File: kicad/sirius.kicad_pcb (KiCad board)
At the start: 4 copper layers, 31.2 x 65.4 mm, 56 parts, among them J1 IPEX_MHF1, J2 Power In, J3 Screw_Terminal, Q1 Q_PMOS_GSD, Q2 Q_NMOS_GSD, Q3 Q_NMOS_GSD, U1 Power_Connector, U2 AP63301WU-7, U3 RFM95W-915S2, U4 LC29H (DA), U5 Pi Zero 2W

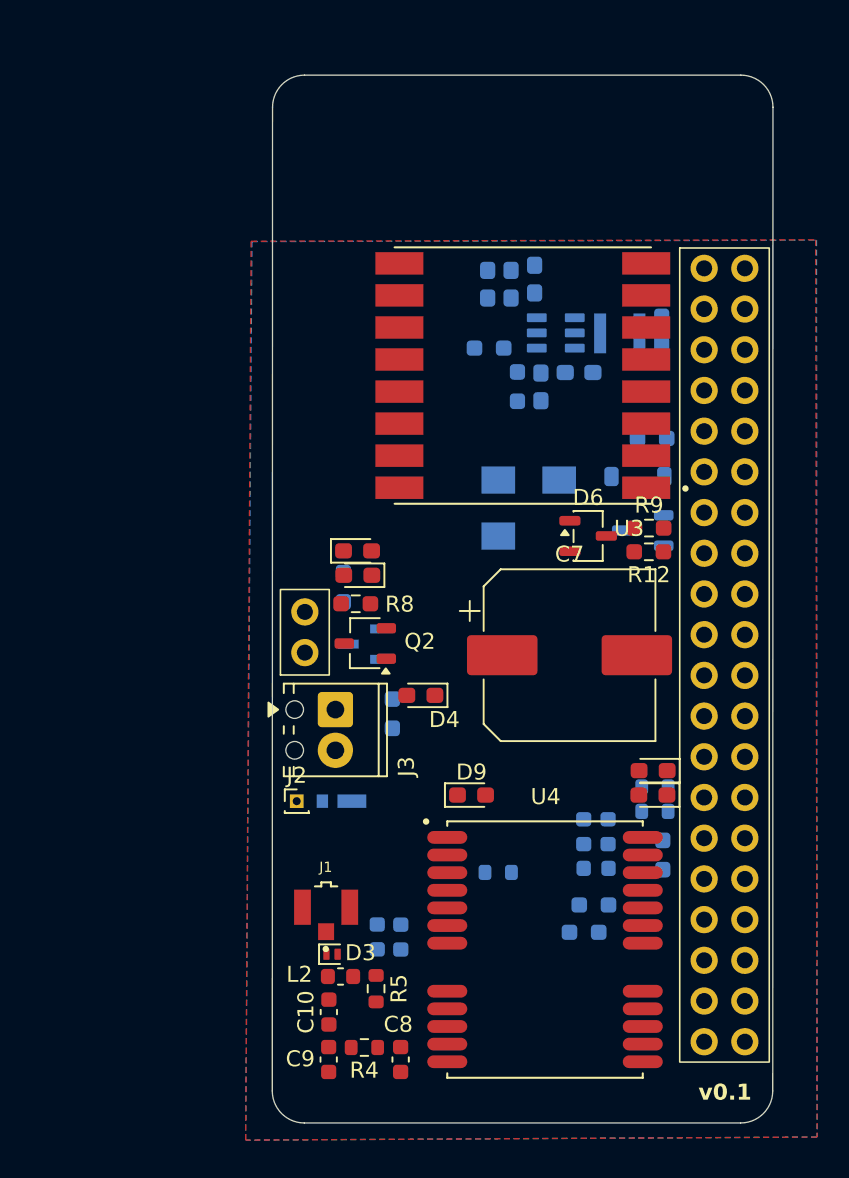
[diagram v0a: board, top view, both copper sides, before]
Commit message: Refactor to use classes properly
Recompile openEMS with boost 1.90 and link wheels. Also update the PCB with the antenna. Still unrouted
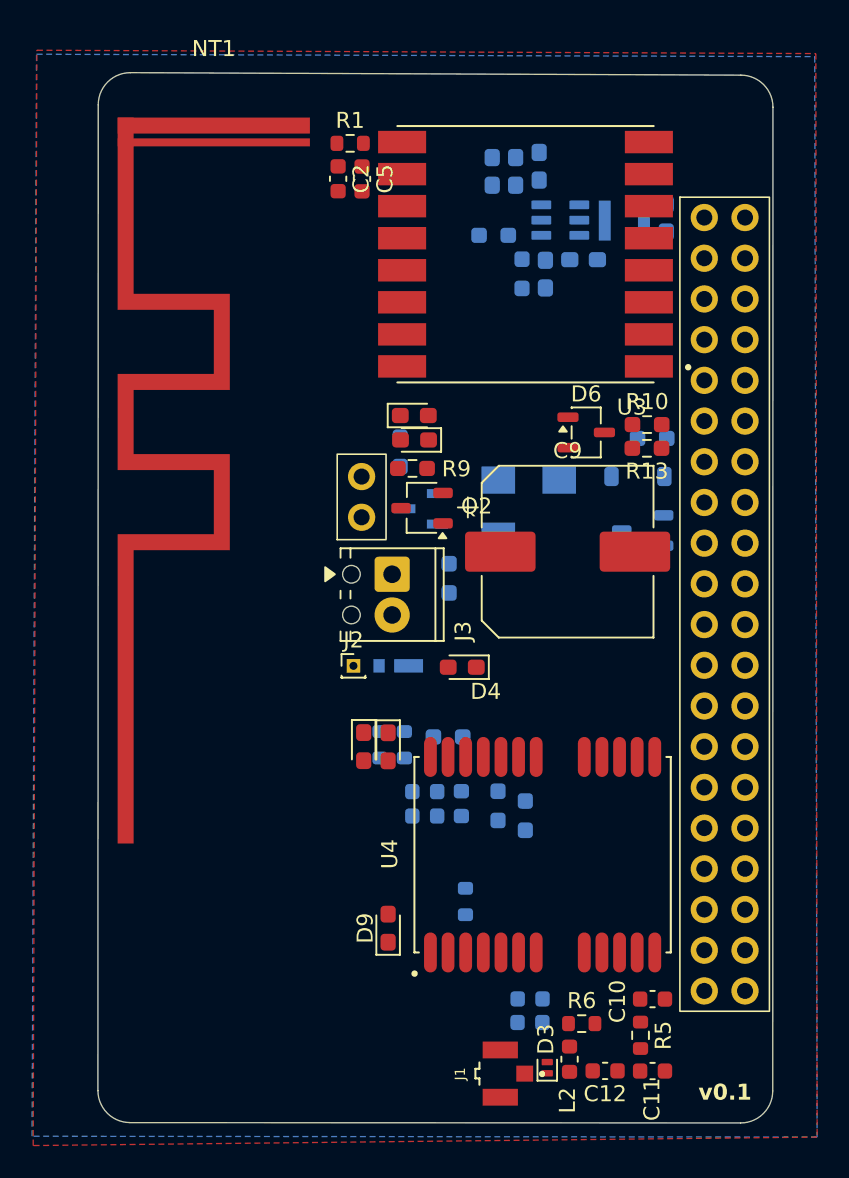
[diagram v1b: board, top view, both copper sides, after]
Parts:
- added C2: 0, Capacitor_SMD:C_0603_1608Metric, F.Cu at (128.1, 72.9)
- added C5: 0, Capacitor_SMD:C_0603_1608Metric, F.Cu at (129.6, 72.9)
- added NT1: NetTie_2, sirius:IFA_915, F.Cu at (120.3, 69.6)
- added R1: 0, Resistor_SMD:R_0603_1608Metric, F.Cu at (128.8, 70.7)
- U3: value RFM95W-915S2 -> XCVR_RFM95W-915S2
- moved C11 20.2 mm to (147.7, 128.6), turned to 180 degrees
- moved D8 18.1 mm to (129.7, 108.4), turned to -90 degrees
- moved C12 17.6 mm to (144.7, 128.6), turned to 180 degrees
- moved R16 17.4 mm to (130.7, 108.2), turned to 90 degrees
- moved R5 17.2 mm to (146.9, 126.4), turned to -90 degrees
- moved D7 16.8 mm to (131.2, 108.4), turned to -90 degrees
- moved R15 16.2 mm to (132.2, 108.2), turned to 90 degrees
- moved C10 16.2 mm to (147.7, 124.1), turned to 180 degrees
- moved R14 15.3 mm to (134.9, 107.8), turned to 180 degrees
- moved L2 15.2 mm to (142.5, 127.9), turned to 90 degrees
- moved D3 15.2 mm to (141.1, 128.4), turned to 90 degrees
- moved J1 15.0 mm to (138.2, 128.8), turned to 90 degrees
- moved R6 13.0 mm to (143.3, 125.6), turned to 0 degrees
- moved C16 11.7 mm to (133.5, 111.2), turned to 0 degrees
- moved C14 10.9 mm to (140.0, 125.6), turned to 180 degrees
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- renumbered C8 to C10, C9 to C11, C10 to C12, C11 to C13, C12 to C14, C13 to C15, C14 to C16, C15 to C17, C2 to C3, C3 to C4, C4 to C6, C5 to C7, C6 to C8, C7 to C9, R9 to R10, R10 to R11, R11 to R12, R12 to R13, R13 to R14, R14 to R15, R15 to R16, R16 to R17, R1 to R2, R2 to R3, R3 to R4, R4 to R5, R5 to R6, R6 to R7, R7 to R8, R8 to R9
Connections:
- U3 pad 9: unconnected-(U3-ANT-Pad9) -> Net-(U3-ANT)
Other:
- board size 31.2 x 65.4 mm -> 42.1 x 65.5 mm
